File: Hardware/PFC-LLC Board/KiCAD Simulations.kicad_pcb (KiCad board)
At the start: 2 copper layers, 210.8 x 69.6 mm, 42 parts, among them J1 1792229, J2 Conn_01x02_Female, J3 1792229, Q1 C2M0160120D, U1 UCC28180DR

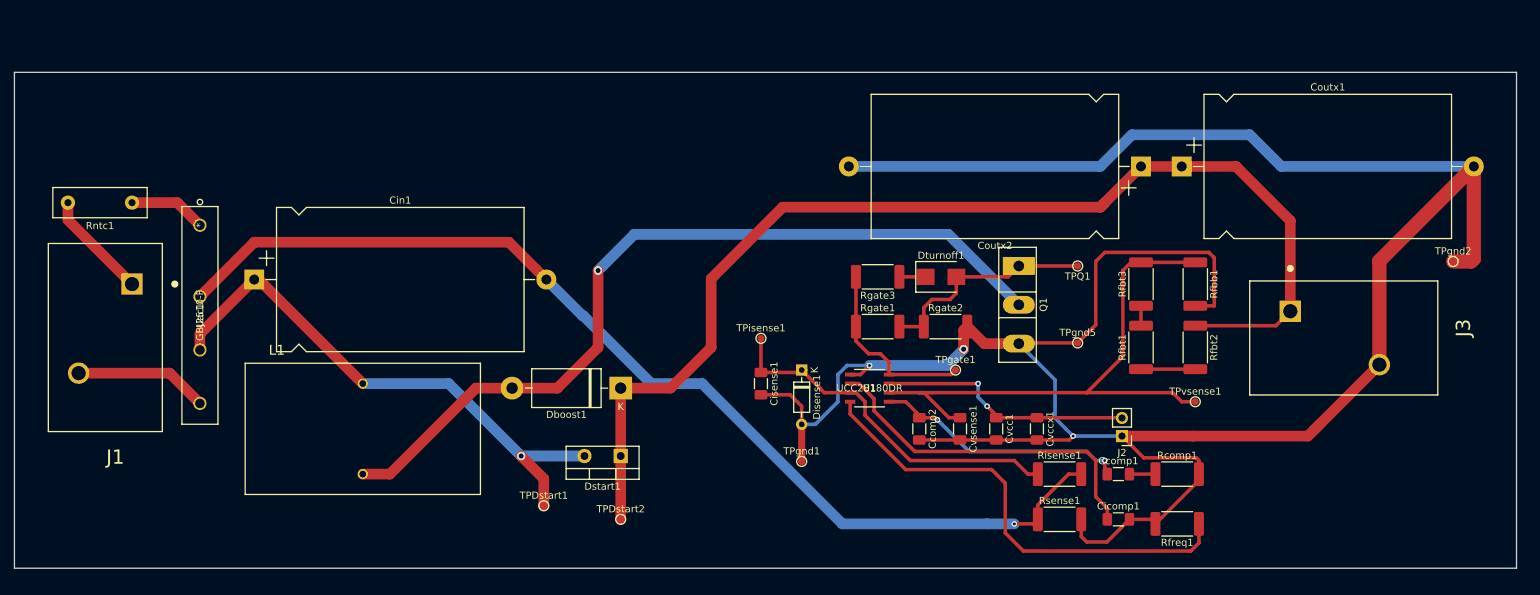
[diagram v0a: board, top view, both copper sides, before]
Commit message: Gerber files regenerated
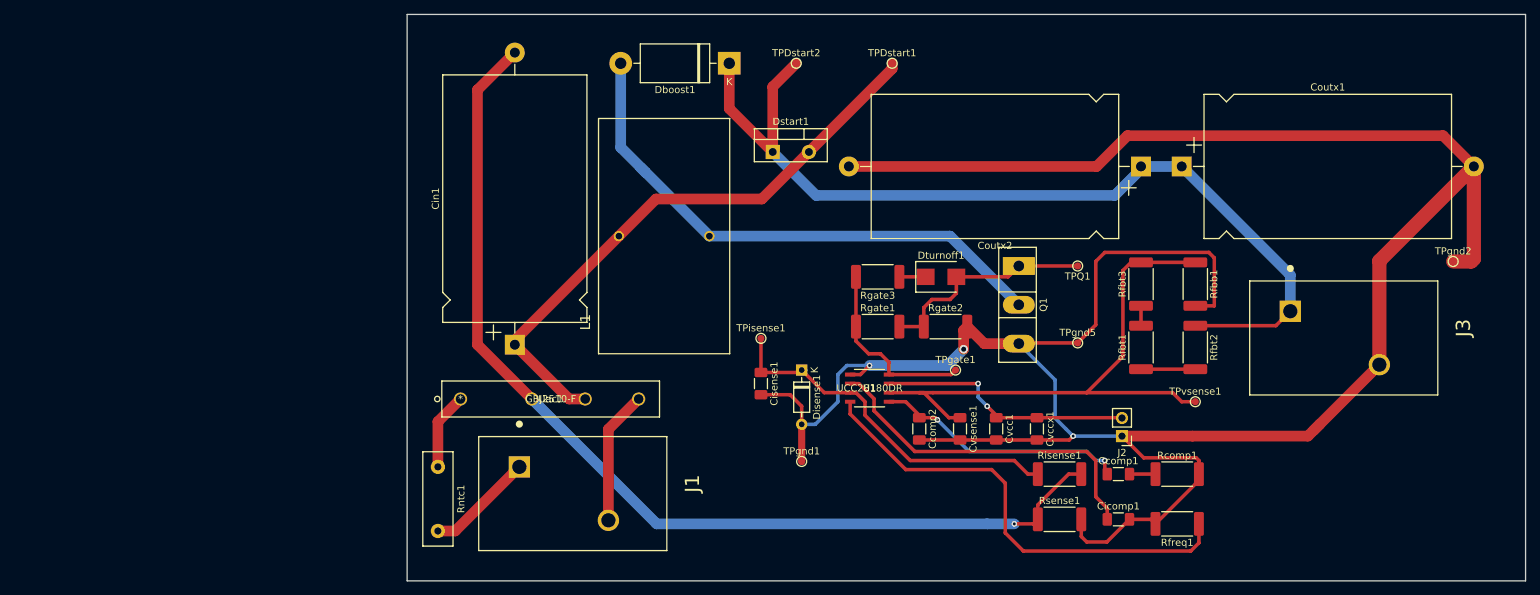
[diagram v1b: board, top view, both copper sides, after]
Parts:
- moved TPDstart1 79.0 mm to (158.8, 26.4)
- moved TPDstart2 68.6 mm to (145.3, 26.4)
- moved J1 60.1 mm to (106.4, 83.1), turned to 270 degrees
- moved Rntc1 56.7 mm to (95.0, 83.1), turned to 270 degrees
- moved L1 50.2 mm to (126.7, 50.7), turned to 90 degrees
- moved Dboost1 48.1 mm to (135.9, 26.4)
- moved Dstart1 47.7 mm to (142.0, 38.9), turned to 0 degrees
- moved Uac1 44.0 mm to (98.2, 73.5), turned to 0 degrees
- moved Cin1 37.7 mm to (105.8, 65.9), turned to 90 degrees
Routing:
- net Net-(Dboost1-Pad2): track 116.4 -> 77.8 mm, vias 1 -> 0
- net Net-(Coutx1-Pad1): track 161.9 -> 131.4 mm
- net Net-(Cin1-Pad1): track 77.9 -> 83.2 mm, vias 1 -> 0
- net Net-(Cin1-Pad2): track 147.3 -> 142.4 mm
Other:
- board size 210.8 x 69.6 mm -> 157 x 79.5 mm
